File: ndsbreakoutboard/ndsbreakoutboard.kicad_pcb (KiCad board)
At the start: 2 copper layers, 2 parts, among them J1 Conn_01x17_Female, U1 ndsPADS

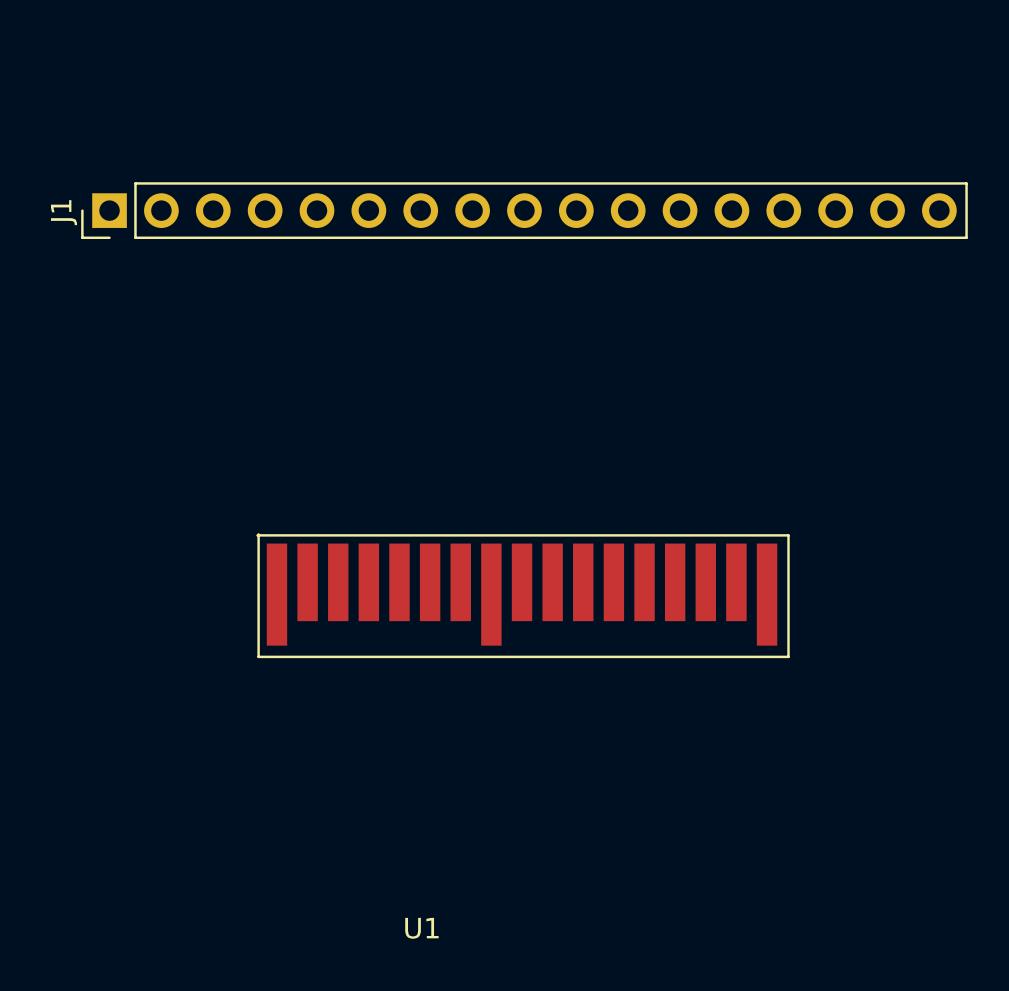
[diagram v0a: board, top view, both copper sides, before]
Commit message: Commit before rebuilding netlist with pin headers
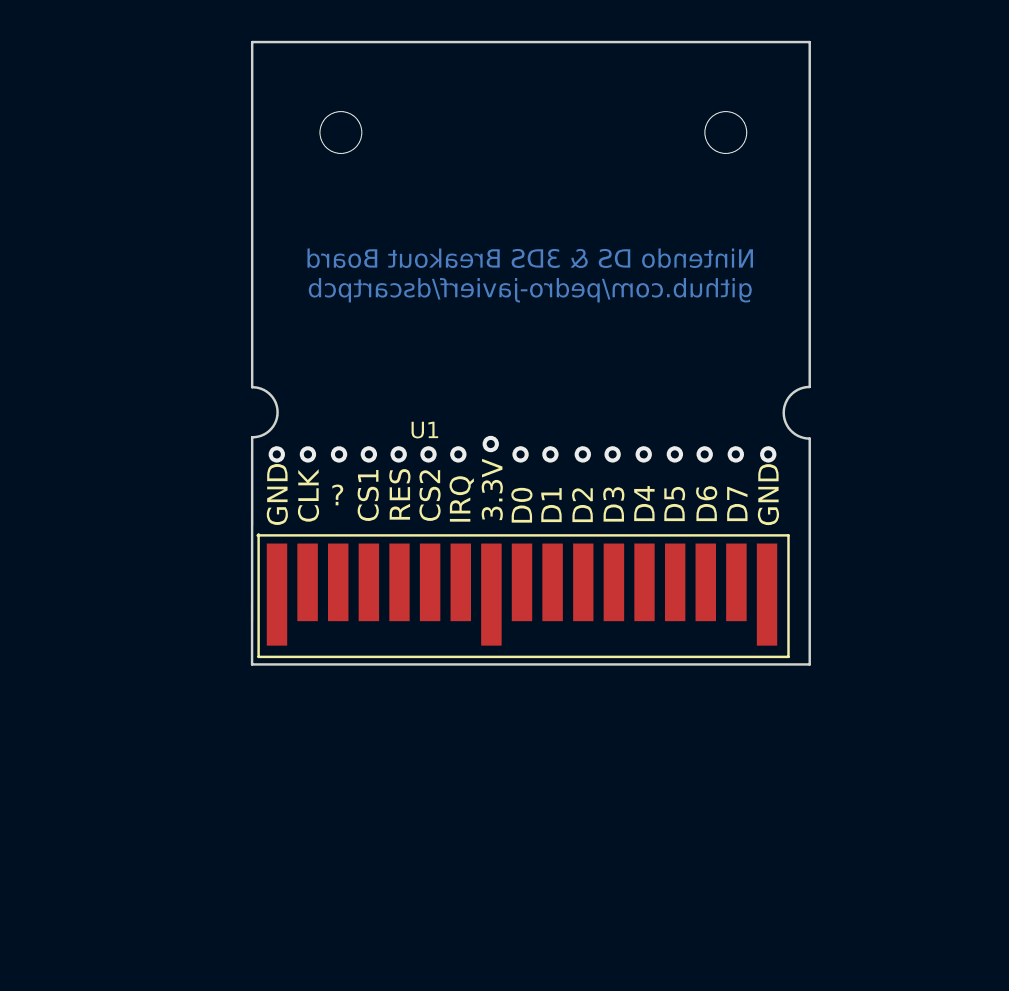
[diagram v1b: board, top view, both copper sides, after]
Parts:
- removed J1: Conn_01x17_Female, Connector_PinHeader_2.54mm:PinHeader_1x17_P2.54mm_Vertical
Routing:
- net (no net): vias 0 -> 19
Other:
- board outline added: 27.3 x 30.5 mm
- board text added: "3.3V"
- board text added: "?"
- board text added: "CLK"
- board text added: "CS1"
- board text added: "CS2"
- board text added: "D0"
- board text added: "D1"
- board text added: "D2"
- board text added: "D3"
- board text added: "D4"
- board text added: "D5"
- board text added: "D6"
- board text added: "D7"
- board text added: "GND"
- board text added: "IRQ"
- board text added: "Nintendo DS & 3DS Breakout Board github.com/pedro-javierf/dscartpcb"
- board text added: "RES"
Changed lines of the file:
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@@
   (general
     (thickness 1.6)
-    (drawings 0)
-    (tracks 0)
+    (drawings 26)
+    (tracks 19)
     (zones 0)
-    (modules 2)
+    (modules 1)
     (nets 18)
   )
@@
     (47 F.CrtYd user)
     (48 B.Fab user)
-    (49 F.Fab user)
+    (49 F.Fab user hide)
   )
   (setup
@@
     (mod_text_size 1 1)
     (mod_text_width 0.15)
-    (pad_size 1.524 1.524)
-    (pad_drill 0.762)
+    (pad_size 0.85 0.85)
+    (pad_drill 0)
     (pad_to_mask_clearance 0.051)
     (solder_mask_min_width 0.25)
@@
     (add_net "Net-(J1-Pad9)")
   )
-  (module Connector_PinHeader_2.54mm:PinHeader_1x17_P2.54mm_Vertical (layer F.Cu)
-    (at 77.47 69.85 90)
-    (descr "Through hole straight pin header, 1x17, 2.54mm pitch, single row")
-    (tags "Through hole pin header THT 1x17 2.54mm single row")
-    (fp_text reference J1 (at 0 -2.33 90) (layer F.SilkS)
-      (effects (font (size 1 1) (thickness 0.15)))
-    )
-    (fp_text value Conn_01x17_Female (at 0 42.97 90) (layer F.Fab)
-      (effects (font (size 1 1) (thickness 0.15)))
-    )
-    (fp_line (start -0.635 -1.27) (end 1.27 -1.27) (layer F.Fab) (width 0.1))
-    (fp_line (start 1.27 -1.27) (end 1.27 41.91) (layer F.Fab) (width 0.1))
-    (fp_line (start 1.27 41.91) (end -1.27 41.91) (layer F.Fab) (width 0.1))
-    (fp_line (start -1.27 41.91) (end -1.27 -0.635) (layer F.Fab) (width 0.1))
-    (fp_line (start -1.27 -0.635) (end -0.635 -1.27) (layer F.Fab) (width 0.1))
-    (fp_line (start -1.33 41.97) (end 1.33 41.97) (layer F.SilkS) (width 0.12))
-    (fp_line (start -1.33 1.27) (end -1.33 41.97) (layer F.SilkS) (width 0.12))
-    (fp_line (start 1.33 1.27) (end 1.33 41.97) (layer F.SilkS) (width 0.12))
-    (fp_line (start -1.33 1.27) (end 1.33 1.27) (layer F.SilkS) (width 0.12))
-    (fp_line (start -1.33 0) (end -1.33 -1.33) (layer F.SilkS) (width 0.12))
-    (fp_line (start -1.33 -1.33) (end 0 -1.33) (layer F.SilkS) (width 0.12))
-    (fp_line (start -1.8 -1.8) (end -1.8 42.45) (layer F.CrtYd) (width 0.05))
-    (fp_line (start -1.8 42.45) (end 1.8 42.45) (layer F.CrtYd) (width 0.05))
-    (fp_line (start 1.8 42.45) (end 1.8 -1.8) (layer F.CrtYd) (width 0.05))
-    (fp_line (start 1.8 -1.8) (end -1.8 -1.8) (layer F.CrtYd) (width 0.05))
-    (fp_text user %R (at 0 20.32) (layer F.Fab)
-      (effects (font (size 1 1) (thickness 0.15)))
-    )
-    (pad 1 thru_hole rect (at 0 0 90) (size 1.7 1.7) (drill 1) (layers *.Cu *.Mask)
-      (net 1 "Net-(J1-Pad1)"))
-    (pad 2 thru_hole oval (at 0 2.54 90) (size 1.7 1.7) (drill 1) (layers *.Cu *.Mask)
-      (net 2 "Net-(J1-Pad2)"))
-    (pad 3 thru_hole oval (at 0 5.08 90) (size 1.7 1.7) (drill 1) (layers *.Cu *.Mask)
-      (net 3 "Net-(J1-Pad3)"))
-    (pad 4 thru_hole oval (at 0 7.62 90) (size 1.7 1.7) (drill 1) (layers *.Cu *.Mask)
-      (net 4 "Net-(J1-Pad4)"))
-    (pad 5 thru_hole oval (at 0 10.16 90) (size 1.7 1.7) (drill 1) (layers *.Cu *.Mask)
-      (net 5 "Net-(J1-Pad5)"))
-    (pad 6 thru_hole oval (at 0 12.7 90) (size 1.7 1.7) (drill 1) (layers *.Cu *.Mask)
-      (net 6 "Net-(J1-Pad6)"))
-    (pad 7 thru_hole oval (at 0 15.24 90) (size 1.7 1.7) (drill 1) (layers *.Cu *.Mask)
-      (net 7 "Net-(J1-Pad7)"))
-    (pad 8 thru_hole oval (at 0 17.78 90) (size 1.7 1.7) (drill 1) (layers *.Cu *.Mask)
-      (net 8 "Net-(J1-Pad8)"))
-    (pad 9 thru_hole oval (at 0 20.32 90) (size 1.7 1.7) (drill 1) (layers *.Cu *.Mask)
-      (net 9 "Net-(J1-Pad9)"))
-    (pad 10 thru_hole oval (at 0 22.86 90) (size 1.7 1.7) (drill 1) (layers *.Cu *.Mask)
-      (net 10 "Net-(J1-Pad10)"))
-    (pad 11 thru_hole oval (at 0 25.4 90) (size 1.7 1.7) (drill 1) (layers *.Cu *.Mask)
-      (net 11 "Net-(J1-Pad11)"))
-    (pad 12 thru_hole oval (at 0 27.94 90) (size 1.7 1.7) (drill 1) (layers *.Cu *.Mask)
-      (net 12 "Net-(J1-Pad12)"))
-    (pad 13 thru_hole oval (at 0 30.48 90) (size 1.7 1.7) (drill 1) (layers *.Cu *.Mask)
-      (net 13 "Net-(J1-Pad13)"))
-    (pad 14 thru_hole oval (at 0 33.02 90) (size 1.7 1.7) (drill 1) (layers *.Cu *.Mask)
-      (net 14 "Net-(J1-Pad14)"))
-    (pad 15 thru_hole oval (at 0 35.56 90) (size 1.7 1.7) (drill 1) (layers *.Cu *.Mask)
-      (net 15 "Net-(J1-Pad15)"))
-    (pad 16 thru_hole oval (at 0 38.1 90) (size 1.7 1.7) (drill 1) (layers *.Cu *.Mask)
-      (net 16 "Net-(J1-Pad16)"))
-    (pad 17 thru_hole oval (at 0 40.64 90) (size 1.7 1.7) (drill 1) (layers *.Cu *.Mask)
-      (net 17 "Net-(J1-Pad17)"))
-    (model ${KISYS3DMOD}/Connector_PinHeader_2.54mm.3dshapes/PinHeader_1x17_P2.54mm_Vertical.wrl
-      (at (xyz 0 0 0))
-      (scale (xyz 1 1 1))
-      (rotate (xyz 0 0 0))
-    )
-  )
   (module Connector:nds_contact_pads (layer F.Cu)
     (at 92.770001 84.705)
     (descr "A footprint for the bottom pads of the NDS cartridge")
     (tags "nds nintendo ds 3ds dsi pads bottom cart card")
-    (fp_text reference U1 (at 0 20.32) (layer F.SilkS)
-      (effects (font (size 1 1) (thickness 0.15)))
+    (fp_text reference U1 (at 0.143199 -4.0854) (layer F.SilkS)
+      (effects (font (size 0.8 0.8) (thickness 0.15)))
     )
-    (fp_text value ndsPADS (at 0 -0.5) (layer F.Fab)
+    (fp_text value ndsPADS (at 5.019999 -5.33) (layer F.Fab)
       (effects (font (size 1 1) (thickness 0.15)))
     )
@@
       (net 17 "Net-(J1-Pad17)"))
   )
+  (gr_text "Nintendo DS & 3DS Breakout Board\ngithub.com/pedro-javierf/dscartpcb" (at 98.075 72.95) (layer B.Cu)
+    (effects (font (size 0.9 0.9) (thickness 0.15)) (justify mirror))
+  )
+  (gr_line (start 84.455 80.9498) (end 84.45 92.075) (layer Edge.Cuts) (width 0.12))
+  (gr_arc (start 84.475 79.725) (end 84.455 80.9498) (angle -181.8343179) (layer Edge.Cuts) (width 0.12))
+  (gr_line (start 111.76 78.486) (end 111.76 61.595) (layer Edge.Cuts) (width 0.12))
+  (gr_arc (start 111.75 79.75) (end 111.76 78.486) (angle -180.9026615) (layer Edge.Cuts) (width 0.12))
+  (gr_text D7 (at 108.25 84.225 90) (layer F.SilkS)
+    (effects (font (size 1 1) (thickness 0.15)))
+  )
+  (gr_text D6 (at 106.75 84.225 90) (layer F.SilkS)
+    (effects (font (size 1 1) (thickness 0.15)))
+  )
+  (gr_text D5 (at 105.175 84.225 90) (layer F.SilkS)
+    (effects (font (size 1 1) (thickness 0.15)))
+  )
+  (gr_text D4 (at 103.7 84.225 90) (layer F.SilkS)
+    (effects (font (size 1 1) (thickness 0.15)))
+  )
+  (gr_text D3 (at 102.2 84.25 90) (layer F.SilkS)
+    (effects (font (size 1 1) (thickness 0.15)))
+  )
+  (gr_text D2 (at 100.675 84.275 90) (layer F.SilkS)
+    (effects (font (size 1 1) (thickness 0.15)))
+  )
+  (gr_text D1 (at 99.15 84.275 90) (layer F.SilkS)
+    (effects (font (size 1 1) (thickness 0.15)))
+  )
+  (gr_text D0 (at 97.7 84.3 90) (layer F.SilkS)
+    (effects (font (size 1 1) (thickness 0.15)))
+  )
+  (gr_text 3.3V (at 96.25 83.55 90) (layer F.SilkS)
+    (effects (font (size 1 1) (thickness 0.15)))
+  )
+  (gr_text IRQ (at 94.675 84 90) (layer F.SilkS)
+    (effects (font (size 1 1) (thickness 0.15)))
+  )
+  (gr_text CS2 (at 93.2 83.775 90) (layer F.SilkS)
+    (effects (font (size 1 1) (thickness 0.15)))
+  )
+  (gr_text RES (at 91.725 83.775 90) (layer F.SilkS)
+    (effects (font (size 1 1) (thickness 0.15)))
+  )
+  (gr_text CS1 (at 90.175 83.775 90) (layer F.SilkS)
+    (effects (font (size 1 1) (thickness 0.15)))
+  )
+  (gr_text ? (at 88.646 83.82) (layer F.SilkS)
+    (effects (font (size 1 1) (thickness 0.15)))
+  )
+  (gr_text CLK (at 87.25 83.85 90) (layer F.SilkS)
+    (effects (font (size 1 1) (thickness 0.15)))
+  )
+  (gr_text GND (at 109.775 83.7565 90) (layer F.SilkS)
+    (effects (font (size 1 1) (thickness 0.15)))
+  )
+  (gr_text GND (at 85.725 83.75 90) (layer F.SilkS)
+    (effects (font (size 1 1) (thickness 0.15)))
+  )
+  (gr_line (start 84.455 61.595) (end 84.455785 78.500187) (layer Edge.Cuts) (width 0.12))
+  (gr_line (start 111.76 61.595) (end 84.455 61.595) (layer Edge.Cuts) (width 0.12))
+  (gr_line (start 111.76 92.075) (end 111.759914 81.014001) (layer Edge.Cuts) (width 0.12))
+  (gr_line (start 84.45 92.075) (end 111.76 92.075) (layer Edge.Cuts) (width 0.12))
+  (via (at 85.6615 81.788) (size 0.8) (drill 0.4) (layers F.Cu B.Cu) (net 0))
+  (via (at 87.1855 81.788) (size 0.8) (drill 0.4) (layers F.Cu B.Cu) (net 0))
+  (via (at 88.7095 81.788) (size 0.8) (drill 0.4) (layers F.Cu B.Cu) (net 0))
+  (via (at 90.17 81.788) (size 0.8) (drill 0.4) (layers F.Cu B.Cu) (net 0))
+  (via (at 91.6305 81.788) (size 0.8) (drill 0.4) (layers F.Cu B.Cu) (net 0))
+  (via (at 93.091 81.788) (size 0.8) (drill 0.4) (layers F.Cu B.Cu) (net 0))
+  (via (at 94.5515 81.788) (size 0.8) (drill 0.4) (layers F.Cu B.Cu) (net 0))
+  (via (at 96.139 81.28) (size 0.8) (drill 0.4) (layers F.Cu B.Cu) (net 0))
+  (via (at 97.5995 81.788) (size 0.8) (drill 0.4) (layers F.Cu B.Cu) (net 0))
+  (via (at 99.06 81.788) (size 0.8) (drill 0.4) (layers F.Cu B.Cu) (net 0))
+  (via (at 100.6475 81.788) (size 0.8) (drill 0.4) (layers F.Cu B.Cu) (net 0))
+  (via (at 102.108 81.788) (size 0.8) (drill 0.4) (layers F.Cu B.Cu) (net 0))
+  (via (at 103.632 81.788) (size 0.8) (drill 0.4) (layers F.Cu B.Cu) (net 0))
+  (via (at 105.156 81.788) (size 0.8) (drill 0.4) (layers F.Cu B.Cu) (net 0))
+  (via (at 106.6165 81.788) (size 0.8) (drill 0.4) (layers F.Cu B.Cu) (net 0))
+  (via (at 108.1405 81.788) (size 0.8) (drill 0.4) (layers F.Cu B.Cu) (net 0))
+  (via (at 109.728 81.788) (size 0.8) (drill 0.4) (layers F.Cu B.Cu) (net 0))
+  (via (at 107.65 66.025) (size 2.1) (drill 2) (layers F.Cu B.Cu) (net 0))
+  (via (at 88.8 66.025) (size 2.1) (drill 2) (layers F.Cu B.Cu) (net 0))
 )
